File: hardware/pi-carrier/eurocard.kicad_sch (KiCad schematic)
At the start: 58 parts, among them J1 DIN41612_C96_male_ra_molliebus, J2 Console, J3 Console, J5 Conn_02x20_raspberry_pi4B, J9 Conn_02x05_Odd_Even, U1 74LVC1G07, U10 Lite-on LTP747KR, U11 TCAN332DR, U12 MCP2518FD, U2 TCAN332DR, U3 LM1117IMPX-3.3, U4 74LVC2G04, U5 74LVC2G38, U6 STM32F103C8T6, U8 SN74AHCT125PWR, U9 MAX7219CWG, X1 ASE-40.000MHz-LC, X2 ASE-8.000MHz-LC, Y1 ABS07-32.768KHZ-6-T

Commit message: pi-carrier: use vertical JST connectors
Problem: horizontal JST connectors are inappropriate for the
design now that less board space is available.

Switch to vertical JST connectors.
Add 3d model.
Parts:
- J2, J3: footprint Connector_JST:JST_SH_SM03B-SRSS-TB_1x03-1MP_P1.00mm_Horizontal -> Connector_JST:JST_SH_BM03B-SRSS-TB_1x03-1MP_P1.00mm_Vertical
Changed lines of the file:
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@@
       (effects (font (size 1.27 1.27)) (justify left) hide)
     )
-    (property "Footprint" "Connector_JST:JST_SH_SM03B-SRSS-TB_1x03-1MP_P1.00mm_Horizontal" (at 255.27 116.84 0)
+    (property "Footprint" "Connector_JST:JST_SH_BM03B-SRSS-TB_1x03-1MP_P1.00mm_Vertical" (at 255.27 116.84 0)
       (effects (font (size 1.27 1.27)) hide)
     )
@@
       (effects (font (size 1.27 1.27)) (justify left) hide)
     )
-    (property "Footprint" "Connector_JST:JST_SH_SM03B-SRSS-TB_1x03-1MP_P1.00mm_Horizontal" (at 255.27 95.25 0)
+    (property "Footprint" "Connector_JST:JST_SH_BM03B-SRSS-TB_1x03-1MP_P1.00mm_Vertical" (at 255.27 95.25 0)
       (effects (font (size 1.27 1.27)) hide)
     )

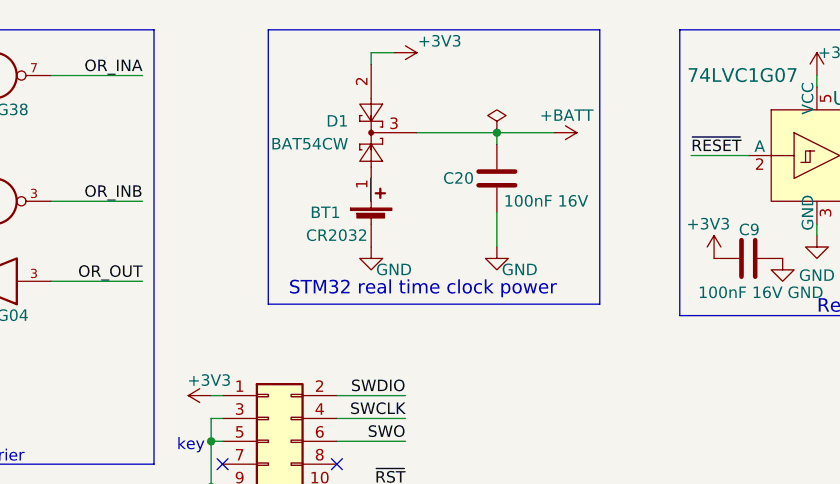
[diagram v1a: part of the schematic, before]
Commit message: pi-carrier: relocate battery, add connectors
Problem: there is no room for an efuse near power entry.

Move the coin battery holder to the other side of the M.2 power
suply and instead of routing, use a JST SH connector that would
allow it to be used either for the STM32 or for a Pi 5 RTC.
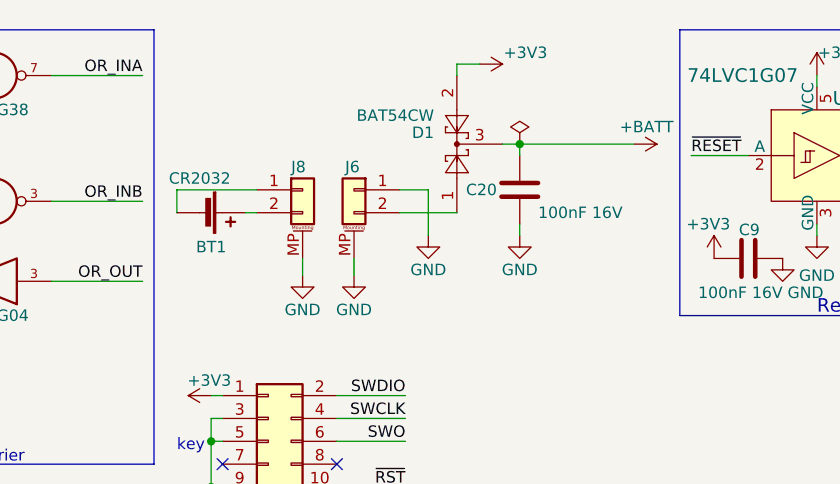
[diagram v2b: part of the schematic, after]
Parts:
- added J6, J8: Conn_01x02_MountingPin, Connector_JST:JST_SH_BM02B-SRSS-TB_1x02-1MP_P1.00mm_Vertical, symbol Connector_Generic_MountingPin:Conn_01x02_MountingPin
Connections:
- net GND: now also J6.1 (Pin_1), J6.MP (MountPin), J8.MP (MountPin); no longer BT1.2 (-)
- net at BT1.1 (+): now also J8.2 (Pin_2); no longer D1.1
- new net: BT1.2 (-), J8.1 (Pin_1)
- new net: D1.1, J6.2 (Pin_2)
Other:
- note removed: "STM32 real time clock power"
- moved on the sheet: BT1, C20, D1
